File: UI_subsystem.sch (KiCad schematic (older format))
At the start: 21 parts

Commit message: relinked LED and BTN footprints. Need to make flash symbol again
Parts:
- BB_BTN_301, BB_BTN_302, ZNP_BTN_301, ZNP_BTN_302: footprint (none) -> Button_Switch_SMD:SW_Push_1P1T_NO_Vertical_Wuerth_434133025816
- BB_L_301, BB_L_302, MCU_L_301, MCU_L_302, PWR301: footprint (none) -> LED_SMD:LED_0603_1608Metric_Pad1.05x0.95mm_HandSolder
- renumbered ZNP_RESET301 to ZNP_RESET1
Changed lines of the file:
@@
 F 0 "ZNP_BTN_301" H 7650 2735 50  0000 C CNN
 F 1 "SW_Push" H 7650 2644 50  0000 C CNN
-F 2 "" H 7650 2650 50  0001 C CNN
+F 2 "Button_Switch_SMD:SW_Push_1P1T_NO_Vertical_Wuerth_434133025816" H 7650 2650 50  0001 C CNN
 F 3 "~" H 7650 2650 50  0001 C CNN
 	1    7650 2450
@@
 F 0 "ZNP_BTN_302" H 8400 2735 50  0000 C CNN
 F 1 "SW_Push" H 8400 2644 50  0000 C CNN
-F 2 "" H 8400 2650 50  0001 C CNN
+F 2 "Button_Switch_SMD:SW_Push_1P1T_NO_Vertical_Wuerth_434133025816" H 8400 2650 50  0001 C CNN
 F 3 "~" H 8400 2650 50  0001 C CNN
 	1    8400 2450
@@
 F 0 "BB_BTN_301" H 9150 2735 50  0000 C CNN
 F 1 "SW_Push" H 9150 2644 50  0000 C CNN
-F 2 "" H 9150 2650 50  0001 C CNN
+F 2 "Button_Switch_SMD:SW_Push_1P1T_NO_Vertical_Wuerth_434133025816" H 9150 2650 50  0001 C CNN
 F 3 "~" H 9150 2650 50  0001 C CNN
 	1    9150 2450
@@
 F 0 "BB_BTN_302" H 9900 2735 50  0000 C CNN
 F 1 "SW_Push" H 9900 2644 50  0000 C CNN
-F 2 "" H 9900 2650 50  0001 C CNN
+F 2 "Button_Switch_SMD:SW_Push_1P1T_NO_Vertical_Wuerth_434133025816" H 9900 2650 50  0001 C CNN
 F 3 "~" H 9900 2650 50  0001 C CNN
 	1    9900 2450
@@
 F 0 "PWR301" V 6839 4682 50  0000 R CNN
 F 1 "LED" V 6748 4682 50  0000 R CNN
-F 2 "" H 6800 4800 50  0001 C CNN
+F 2 "LED_SMD:LED_0603_1608Metric_Pad1.05x0.95mm_HandSolder" H 6800 4800 50  0001 C CNN
 F 3 "~" H 6800 4800 50  0001 C CNN
 	1    6800 4800
@@
 F 0 "MCU_L_301" V 7639 4682 50  0000 R CNN
 F 1 "LED" V 7548 4682 50  0000 R CNN
-F 2 "" H 7600 4800 50  0001 C CNN
+F 2 "LED_SMD:LED_0603_1608Metric_Pad1.05x0.95mm_HandSolder" H 7600 4800 50  0001 C CNN
 F 3 "~" H 7600 4800 50  0001 C CNN
 	1    7600 4800
@@
 F 0 "MCU_L_302" V 8489 4682 50  0000 R CNN
 F 1 "LED" V 8398 4682 50  0000 R CNN
-F 2 "" H 8450 4800 50  0001 C CNN
+F 2 "LED_SMD:LED_0603_1608Metric_Pad1.05x0.95mm_HandSolder" H 8450 4800 50  0001 C CNN
 F 3 "~" H 8450 4800 50  0001 C CNN
 	1    8450 4800
@@
 F 0 "BB_L_301" V 9339 4682 50  0000 R CNN
 F 1 "LED" V 9248 4682 50  0000 R CNN
-F 2 "" H 9300 4800 50  0001 C CNN
+F 2 "LED_SMD:LED_0603_1608Metric_Pad1.05x0.95mm_HandSolder" H 9300 4800 50  0001 C CNN
 F 3 "~" H 9300 4800 50  0001 C CNN
 	1    9300 4800
@@
 F 0 "BB_L_302" V 10189 4682 50  0000 R CNN
 F 1 "LED" V 10098 4682 50  0000 R CNN
-F 2 "" H 10150 4800 50  0001 C CNN
+F 2 "LED_SMD:LED_0603_1608Metric_Pad1.05x0.95mm_HandSolder" H 10150 4800 50  0001 C CNN
 F 3 "~" H 10150 4800 50  0001 C CNN
 	1    10150 4800
@@
 	10200 1450 10200 1600
 $Comp
-L Switch:SW_Push ZNP_RESET301
+L Switch:SW_Push ZNP_RESET1
 U 1 1 614AD723
 P 6900 2450

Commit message: Recovered the .lib for flash symbol. Relinked in schematic
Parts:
- BB_BTN_301, BB_BTN_302, ZNP_BTN_301, ZNP_BTN_302, ZNP_RESET1: symbol Switch:SW_Push -> BeagleBone-Black-Cape-rescue:SW_Push-Switch
- BB_L_301, BB_L_302, MCU_L_301, MCU_L_302, PWR301: symbol Device:LED -> BeagleBone-Black-Cape-rescue:LED-Device
- R301, R302, R303, R304, R305, R306, R307, R308, R309, R310: symbol Device:R_US -> BeagleBone-Black-Cape-rescue:R_US-Device
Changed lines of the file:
@@
 	3150 3550 3300 3550
 $Comp
-L Switch:SW_Push ZNP_BTN_301
+L BeagleBone-Black-Cape-rescue:SW_Push-Switch ZNP_BTN_301
 U 1 1 614536C0
 P 7650 2450
@@
 $EndComp
 $Comp
-L Switch:SW_Push ZNP_BTN_302
+L BeagleBone-Black-Cape-rescue:SW_Push-Switch ZNP_BTN_302
 U 1 1 614542E2
 P 8400 2450
@@
 $EndComp
 $Comp
-L Switch:SW_Push BB_BTN_301
+L BeagleBone-Black-Cape-rescue:SW_Push-Switch BB_BTN_301
 U 1 1 614544C6
 P 9150 2450
@@
 $EndComp
 $Comp
-L Switch:SW_Push BB_BTN_302
+L BeagleBone-Black-Cape-rescue:SW_Push-Switch BB_BTN_302
 U 1 1 61454891
 P 9900 2450
@@
 $EndComp
 $Comp
-L Device:LED PWR301
+L BeagleBone-Black-Cape-rescue:LED-Device PWR301
 U 1 1 614557C3
 P 6800 4800
@@
 $EndComp
 $Comp
-L Device:LED MCU_L_301
+L BeagleBone-Black-Cape-rescue:LED-Device MCU_L_301
 U 1 1 614568E7
 P 7600 4800
@@
 $EndComp
 $Comp
-L Device:LED MCU_L_302
+L BeagleBone-Black-Cape-rescue:LED-Device MCU_L_302
 U 1 1 61456F00
 P 8450 4800
@@
 $EndComp
 $Comp
-L Device:LED BB_L_301
+L BeagleBone-Black-Cape-rescue:LED-Device BB_L_301
 U 1 1 614573C9
 P 9300 4800
@@
 $EndComp
 $Comp
-L Device:LED BB_L_302
+L BeagleBone-Black-Cape-rescue:LED-Device BB_L_302
 U 1 1 61457651
 P 10150 4800
@@
 $EndComp
 $Comp
-L Device:R_US R301
+L BeagleBone-Black-Cape-rescue:R_US-Device R301
 U 1 1 614578E4
 P 6800 4450
@@
 	6800 4950 6800 5100
 $Comp
-L Device:R_US R303
+L BeagleBone-Black-Cape-rescue:R_US-Device R303
 U 1 1 61463DB5
 P 7600 4450
@@
 $EndComp
 $Comp
-L Device:R_US R306
+L BeagleBone-Black-Cape-rescue:R_US-Device R306
 U 1 1 614640E9
 P 8450 4450
@@
 $EndComp
 $Comp
-L Device:R_US R307
+L BeagleBone-Black-Cape-rescue:R_US-Device R307
 U 1 1 614643AB
 P 9300 4450
@@
 $EndComp
 $Comp
-L Device:R_US R309
+L BeagleBone-Black-Cape-rescue:R_US-Device R309
 U 1 1 61464797
 P 10150 4450
@@
 $EndComp
 $Comp
-L Device:R_US R304
+L BeagleBone-Black-Cape-rescue:R_US-Device R304
 U 1 1 61481C85
 P 7650 1950
@@
 Connection ~ 10200 1600
 $Comp
-L Device:R_US R305
+L BeagleBone-Black-Cape-rescue:R_US-Device R305
 U 1 1 61482BE5
 P 8400 1950
@@
 $EndComp
 $Comp
-L Device:R_US R308
+L BeagleBone-Black-Cape-rescue:R_US-Device R308
 U 1 1 614833DA
 P 9450 1900
@@
 $EndComp
 $Comp
-L Device:R_US R310
+L BeagleBone-Black-Cape-rescue:R_US-Device R310
 U 1 1 614839E0
 P 10200 1900
@@
 	10200 1450 10200 1600
 $Comp
-L Switch:SW_Push ZNP_RESET1
+L BeagleBone-Black-Cape-rescue:SW_Push-Switch ZNP_RESET1
 U 1 1 614AD723
 P 6900 2450
@@
 $EndComp
 $Comp
-L Device:R_US R302
+L BeagleBone-Black-Cape-rescue:R_US-Device R302
 U 1 1 614AD729
 P 6900 1950
@@
 	7650 2850 6900 2850
 $Comp
-L power:GND #PWR0301
+L BeagleBone-Black-Cape-rescue:GND-power #PWR0301
 U 1 1 614B24A7
 P 2400 2800

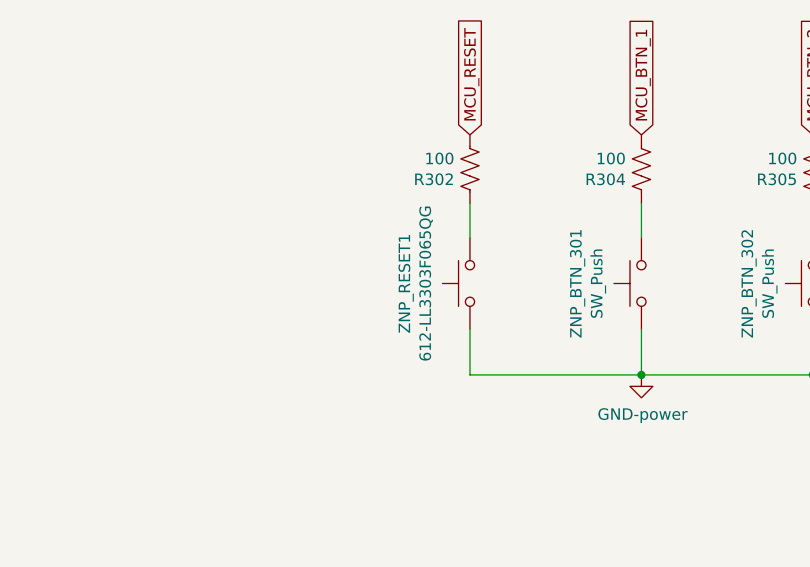
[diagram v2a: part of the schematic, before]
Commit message: prepped for PSU subsystem placements
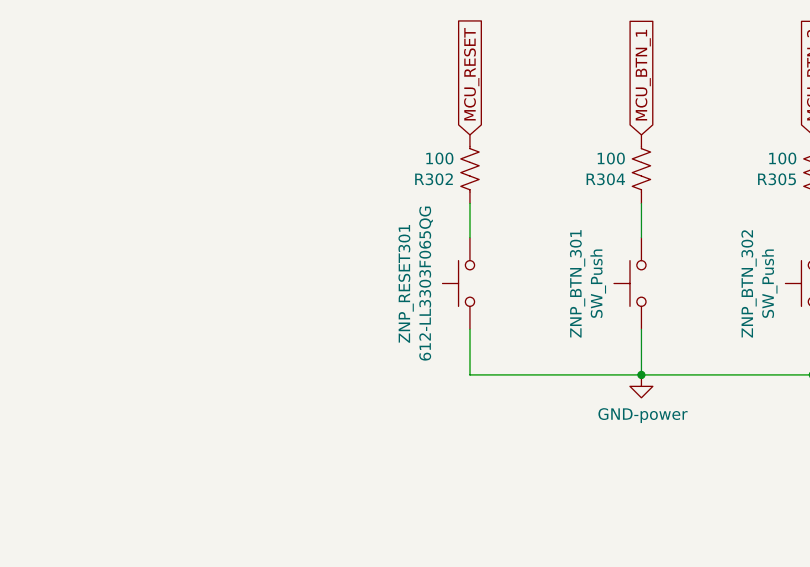
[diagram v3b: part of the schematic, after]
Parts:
- renumbered ZNP_RESET1 to ZNP_RESET301
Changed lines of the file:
@@
 	10200 1450 10200 1600
 $Comp
-L BeagleBone-Black-Cape-rescue:SW_Push-Switch ZNP_RESET1
+L BeagleBone-Black-Cape-rescue:SW_Push-Switch ZNP_RESET301
 U 1 1 614AD723
 P 6900 2450
-F 0 "ZNP_RESET1" H 6900 2735 50  0000 C CNN
+F 0 "ZNP_RESET301" H 6900 2735 50  0000 C CNN
 F 1 "612-LL3303F065QG" H 6900 2644 50  0000 C CNN
 F 2 "Button_Switch_SMD:SW_Push_1P1T_NO_Vertical_Wuerth_434133025816" H 6900 2650 50  0001 C CNN

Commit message: lib update so it only includes user-made library
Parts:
- BB_BTN_301, BB_BTN_302, ZNP_BTN_301, ZNP_BTN_302, ZNP_RESET301: symbol BeagleBone-Black-Cape-rescue:SW_Push-Switch -> UserMade-BB-Zigbee-Gateway-CAPE:SW_Push-Switch
- BB_L_301, BB_L_302, MCU_L_301, MCU_L_302, PWR301: symbol BeagleBone-Black-Cape-rescue:LED-Device -> UserMade-BB-Zigbee-Gateway-CAPE:LED-Device
- R301, R302, R303, R304, R305, R306, R307, R308, R309, R310: symbol BeagleBone-Black-Cape-rescue:R_US-Device -> UserMade-BB-Zigbee-Gateway-CAPE:R_US-Device
- TFT301: symbol cc1352:ST7735_TFT -> UserMade-BB-Zigbee-Gateway-CAPE:ST7735_TFT
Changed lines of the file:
@@
 D.C_TFT
 $Comp
-L cc1352:ST7735_TFT TFT301
+L UserMade-BB-Zigbee-Gateway-CAPE:ST7735_TFT TFT301
 U 1 1 6083DD31
 P 4800 3950
@@
 	3150 3550 3300 3550
 $Comp
-L BeagleBone-Black-Cape-rescue:SW_Push-Switch ZNP_BTN_301
+L UserMade-BB-Zigbee-Gateway-CAPE:SW_Push-Switch ZNP_BTN_301
 U 1 1 614536C0
 P 7650 2450
@@
 $EndComp
 $Comp
-L BeagleBone-Black-Cape-rescue:SW_Push-Switch ZNP_BTN_302
+L UserMade-BB-Zigbee-Gateway-CAPE:SW_Push-Switch ZNP_BTN_302
 U 1 1 614542E2
 P 8400 2450
@@
 $EndComp
 $Comp
-L BeagleBone-Black-Cape-rescue:SW_Push-Switch BB_BTN_301
+L UserMade-BB-Zigbee-Gateway-CAPE:SW_Push-Switch BB_BTN_301
 U 1 1 614544C6
 P 9150 2450
@@
 $EndComp
 $Comp
-L BeagleBone-Black-Cape-rescue:SW_Push-Switch BB_BTN_302
+L UserMade-BB-Zigbee-Gateway-CAPE:SW_Push-Switch BB_BTN_302
 U 1 1 61454891
 P 9900 2450
@@
 $EndComp
 $Comp
-L BeagleBone-Black-Cape-rescue:LED-Device PWR301
+L UserMade-BB-Zigbee-Gateway-CAPE:LED-Device PWR301
 U 1 1 614557C3
 P 6800 4800
@@
 $EndComp
 $Comp
-L BeagleBone-Black-Cape-rescue:LED-Device MCU_L_301
+L UserMade-BB-Zigbee-Gateway-CAPE:LED-Device MCU_L_301
 U 1 1 614568E7
 P 7600 4800
@@
 $EndComp
 $Comp
-L BeagleBone-Black-Cape-rescue:LED-Device MCU_L_302
+L UserMade-BB-Zigbee-Gateway-CAPE:LED-Device MCU_L_302
 U 1 1 61456F00
 P 8450 4800
@@
 $EndComp
 $Comp
-L BeagleBone-Black-Cape-rescue:LED-Device BB_L_301
+L UserMade-BB-Zigbee-Gateway-CAPE:LED-Device BB_L_301
 U 1 1 614573C9
 P 9300 4800
@@
 $EndComp
 $Comp
-L BeagleBone-Black-Cape-rescue:LED-Device BB_L_302
+L UserMade-BB-Zigbee-Gateway-CAPE:LED-Device BB_L_302
 U 1 1 61457651
 P 10150 4800
@@
 $EndComp
 $Comp
-L BeagleBone-Black-Cape-rescue:R_US-Device R301
+L UserMade-BB-Zigbee-Gateway-CAPE:R_US-Device R301
 U 1 1 614578E4
 P 6800 4450
@@
 $EndComp
 $Comp
-L BeagleBone-Black-Cape-rescue:GND-power #PWR0302
+L UserMade-BB-Zigbee-Gateway-CAPE:GND-power #PWR0302
 U 1 1 61458C9B
 P 6800 5200
@@
 	6800 4950 6800 5100
 $Comp
-L BeagleBone-Black-Cape-rescue:R_US-Device R303
+L UserMade-BB-Zigbee-Gateway-CAPE:R_US-Device R303
 U 1 1 61463DB5
 P 7600 4450
@@
 $EndComp
 $Comp
-L BeagleBone-Black-Cape-rescue:R_US-Device R306
+L UserMade-BB-Zigbee-Gateway-CAPE:R_US-Device R306
 U 1 1 614640E9
 P 8450 4450
@@
 $EndComp
 $Comp
-L BeagleBone-Black-Cape-rescue:R_US-Device R307
+L UserMade-BB-Zigbee-Gateway-CAPE:R_US-Device R307
 U 1 1 614643AB
 P 9300 4450
@@
 $EndComp
 $Comp
-L BeagleBone-Black-Cape-rescue:R_US-Device R309
+L UserMade-BB-Zigbee-Gateway-CAPE:R_US-Device R309
 U 1 1 61464797
 P 10150 4450
@@
 	6800 4600 6800 4650
 $Comp
-L BeagleBone-Black-Cape-rescue:GND-power #PWR0303
+L UserMade-BB-Zigbee-Gateway-CAPE:GND-power #PWR0303
 U 1 1 61474E36
 P 7650 2850
@@
 $EndComp
 $Comp
-L BeagleBone-Black-Cape-rescue:R_US-Device R304
+L UserMade-BB-Zigbee-Gateway-CAPE:R_US-Device R304
 U 1 1 61481C85
 P 7650 1950
@@
 Connection ~ 10200 1600
 $Comp
-L BeagleBone-Black-Cape-rescue:R_US-Device R305
+L UserMade-BB-Zigbee-Gateway-CAPE:R_US-Device R305
 U 1 1 61482BE5
 P 8400 1950
@@
 $EndComp
 $Comp
-L BeagleBone-Black-Cape-rescue:R_US-Device R308
+L UserMade-BB-Zigbee-Gateway-CAPE:R_US-Device R308
 U 1 1 614833DA
 P 9450 1900
@@
 $EndComp
 $Comp
-L BeagleBone-Black-Cape-rescue:R_US-Device R310
+L UserMade-BB-Zigbee-Gateway-CAPE:R_US-Device R310
 U 1 1 614839E0
 P 10200 1900
@@
 	10200 1450 10200 1600
 $Comp
-L BeagleBone-Black-Cape-rescue:SW_Push-Switch ZNP_RESET301
+L UserMade-BB-Zigbee-Gateway-CAPE:SW_Push-Switch ZNP_RESET301
 U 1 1 614AD723
 P 6900 2450
@@
 $EndComp
 $Comp
-L BeagleBone-Black-Cape-rescue:R_US-Device R302
+L UserMade-BB-Zigbee-Gateway-CAPE:R_US-Device R302
 U 1 1 614AD729
 P 6900 1950
@@
 	7650 2850 6900 2850
 $Comp
-L BeagleBone-Black-Cape-rescue:GND-power #PWR0301
+L UserMade-BB-Zigbee-Gateway-CAPE:GND-power #PWR0301
 U 1 1 614B24A7
 P 2400 2800

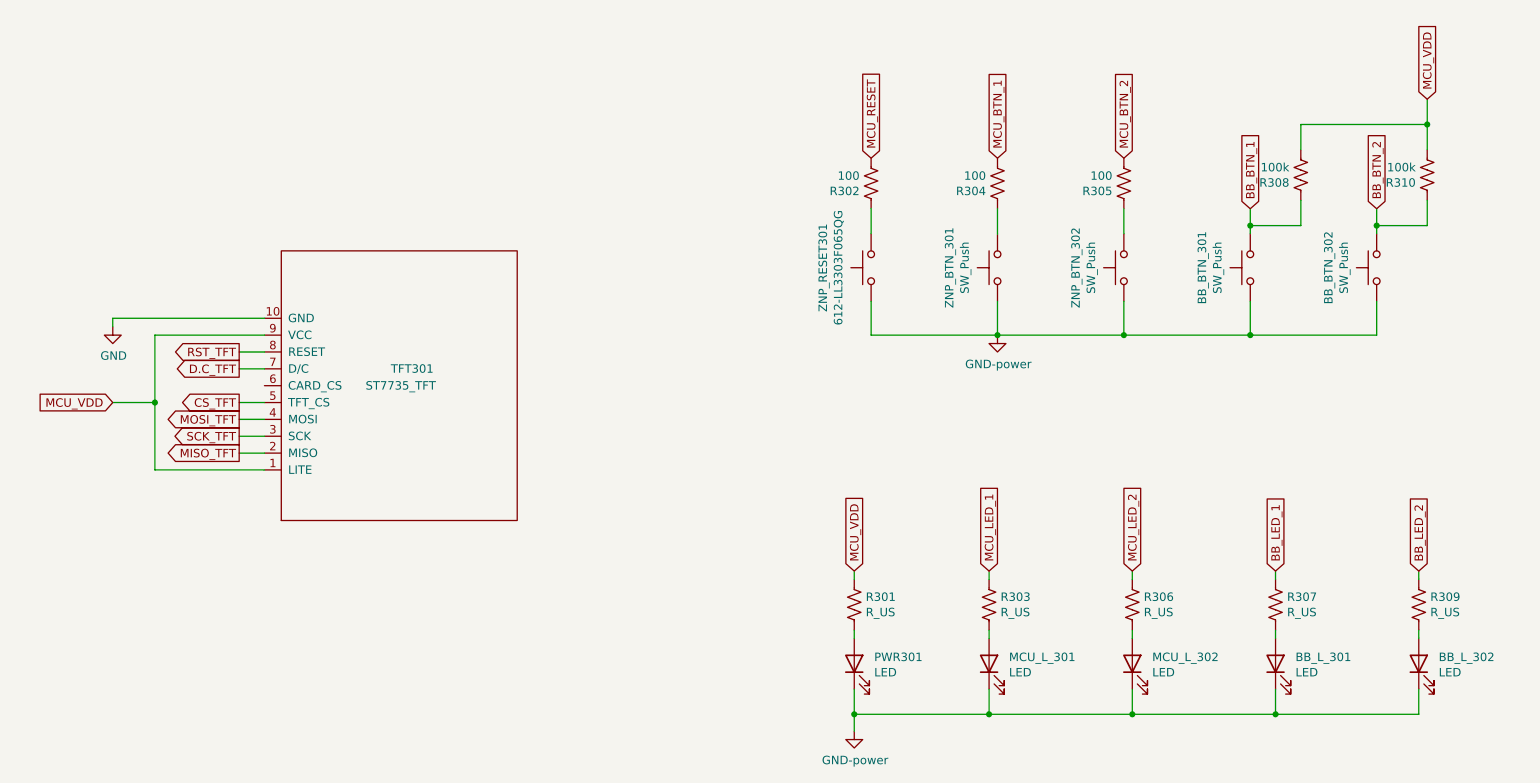
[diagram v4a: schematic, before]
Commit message: final edits before it'll be untouched
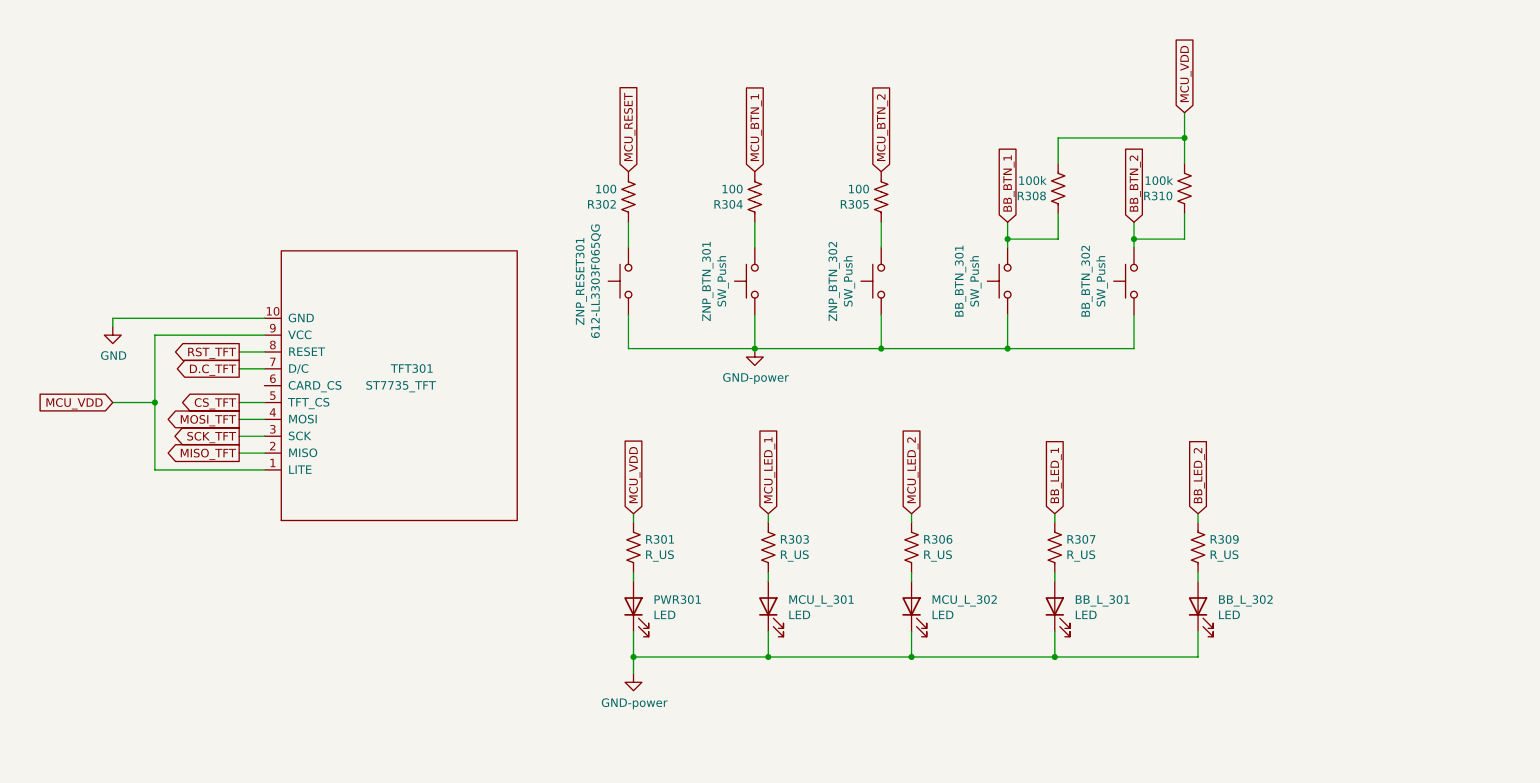
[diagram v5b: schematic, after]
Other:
- moved on the sheet: BB_BTN_301, BB_BTN_302, BB_L_301, BB_L_302, MCU_L_301, MCU_L_302, PWR301, R301, R302, R303, R304, R305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
